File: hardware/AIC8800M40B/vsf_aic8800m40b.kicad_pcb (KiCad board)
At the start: 4 copper layers, 36.8 x 57.2 mm, 92 parts, among them J1 USB_A, J2 USB_C_Receptacle_USB2.0, J3 USB_C_Receptacle_USB2.0, J4 Micro_SD_Card_Det1, J6 Conn_Coaxial, J7 Conn_Coaxial, J8 Conn_02x15_Odd_Even, Q1 S9013, Q2 PMBT3904, SW1 SW_Push, SW2 SW_Push, SW3 SW_Push, SW4 SW_Push, U1 AIC8800MX0_48P, U2 CH340N, U3 ETA9638, U4 ETA3486, Y1 40M, 10PPM,10pF

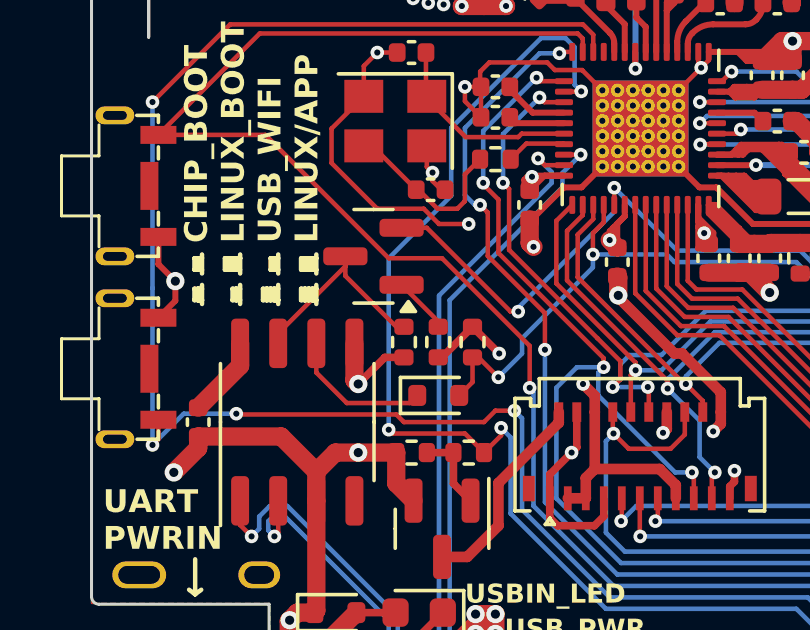
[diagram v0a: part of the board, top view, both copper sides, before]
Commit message: [hardware/aic8800m40b] update
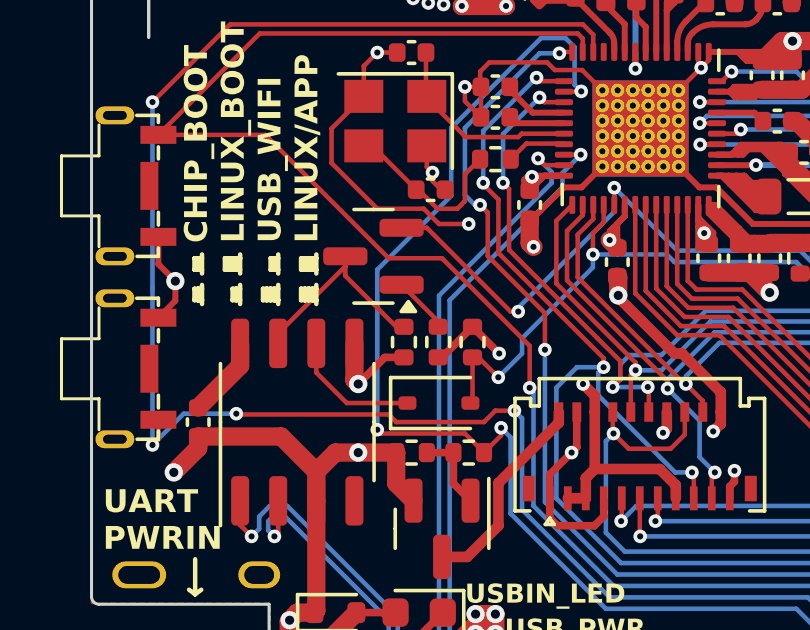
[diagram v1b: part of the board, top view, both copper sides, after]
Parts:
- C30: value 0Ohm -> NC
- D4: value 1N4148 -> PMEG1030EJ; footprint Diode_SMD:D_SOD-523 -> Diode_SMD:D_SOD-323
- R23: value NC -> 0Ohm
- moved D4 0.26 mm to (214.8, 118.2)
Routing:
- net /GPIOB4: track 49.2 -> 49.8 mm
